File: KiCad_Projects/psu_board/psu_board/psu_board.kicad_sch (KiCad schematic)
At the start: 23 parts, among them J1 Conn_01x02_Female, J2 Conn_01x02_Female, J3 Conn_01x02_Female, SW1 SW_DIP_x01, SW2 SW_DIP_x01, U1 OKL-T_6-W12N-C

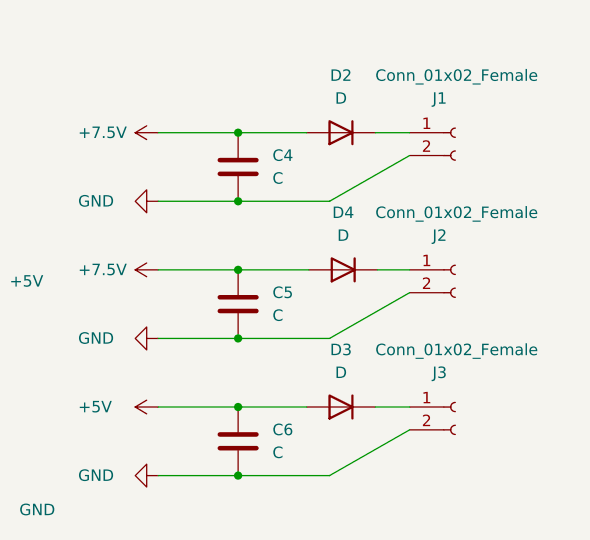
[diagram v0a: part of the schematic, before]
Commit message: 基盤データのアップデート
ローカルコミットはちゃんと作ってください
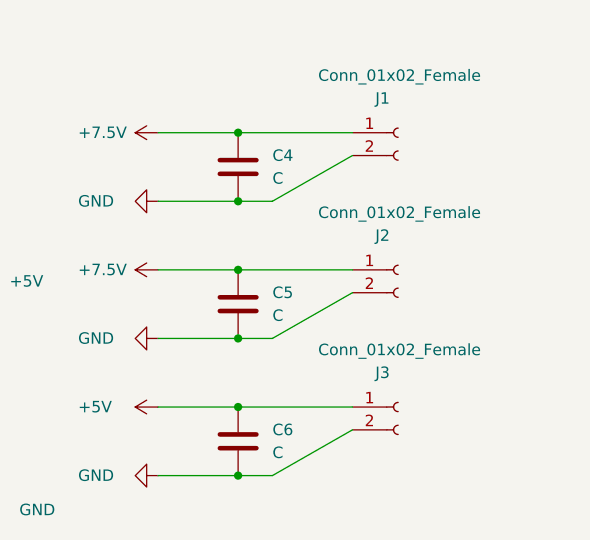
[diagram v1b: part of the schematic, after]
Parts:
- removed D2, D3, D4: D, Diode_THT:D_DO-41_SOD81_P7.62mm_Horizontal, symbol Device:D
- BT1: footprint (none) -> Connector_JST:JST_VH_B2P-VH-B_1x02_P3.96mm_Vertical
- C6: footprint Capacitor_THT:CP_Radial_D5.0mm_P2.50mm -> (none)
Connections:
- net +5V: now also J3.1 (Pin_1)
- net +7.5V: now also J1.1 (Pin_1), J2.1 (Pin_1)
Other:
- moved on the sheet: J1, J2, J3
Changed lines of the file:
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@@
-    (stroke (width 0) (type default) (color 0 0 0 0))
-  )
-  (wire (pts (xy 236.22 110.49) (xy 240.03 110.49))
     (stroke (width 0) (type default) (color 0 0 0 0))
   )
@@
     (stroke (width 0) (type default) (color 0 0 0 0))
   )
-  (wire (pts (xy 220.98 102.87) (xy 231.14 102.87))
-    (stroke (width 0) (type default) (color 0 0 0 0))
-  )
-  (wire (pts (xy 220.98 80.01) (xy 228.6 80.01))
+  (wire (pts (xy 220.98 102.87) (xy 224.79 102.87))
     (stroke (width 0) (type default) (color 0 0 0 0))
   )
@@
     (stroke (width 0) (type default) (color 0 0 0 0))
   )
-  (wire (pts (xy 236.4672 95.25) (xy 240.03 95.25))
-    (stroke (width 0) (type default) (color 0 0 0 0))
-  )
   (wire (pts (xy 109.22 105.41) (xy 109.22 101.6))
     (stroke (width 0) (type default) (color 0 0 0 0))
@@
     (stroke (width 0) (type default) (color 0 0 0 0))
   )
-  (wire (pts (xy 231.14 102.87) (xy 240.03 97.79))
+  (wire (pts (xy 224.79 102.87) (xy 233.68 97.79))
     (stroke (width 0) (type default) (color 0 0 0 0))
   )
@@
     (stroke (width 0) (type default) (color 0 0 0 0))
   )
-  (wire (pts (xy 220.98 110.49) (xy 228.6 110.49))
+  (wire (pts (xy 220.98 110.49) (xy 233.68 110.49))
     (stroke (width 0) (type default) (color 0 0 0 0))
   )
@@
     (stroke (width 0) (type default) (color 0 0 0 0))
   )
-  (wire (pts (xy 231.14 87.63) (xy 240.03 82.55))
+  (wire (pts (xy 224.79 87.63) (xy 233.68 82.55))
     (stroke (width 0) (type default) (color 0 0 0 0))
   )
@@
     (stroke (width 0) (type default) (color 0 0 0 0))
   )
-  (wire (pts (xy 231.14 118.11) (xy 240.03 113.03))
-    (stroke (width 0) (type default) (color 0 0 0 0))
-  )
-  (wire (pts (xy 220.98 95.25) (xy 228.8472 95.25))
+  (wire (pts (xy 224.79 118.11) (xy 233.68 113.03))
+    (stroke (width 0) (type default) (color 0 0 0 0))
+  )
+  (wire (pts (xy 220.98 95.25) (xy 233.68 95.25))
     (stroke (width 0) (type default) (color 0 0 0 0))
   )
@@
     (stroke (width 0) (type default) (color 0 0 0 0))
   )
-  (wire (pts (xy 236.22 80.01) (xy 240.03 80.01))
+  (wire (pts (xy 220.98 80.01) (xy 233.68 80.01))
     (stroke (width 0) (type default) (color 0 0 0 0))
   )
@@
     (stroke (width 0) (type default) (color 0 0 0 0))
   )
-  (wire (pts (xy 220.98 87.63) (xy 231.14 87.63))
+  (wire (pts (xy 220.98 87.63) (xy 224.79 87.63))
     (stroke (width 0) (type default) (color 0 0 0 0))
   )
@@
     (stroke (width 0) (type default) (color 0 0 0 0))
   )
-  (wire (pts (xy 220.98 118.11) (xy 231.14 118.11))
+  (wire (pts (xy 220.98 118.11) (xy 224.79 118.11))
     (stroke (width 0) (type default) (color 0 0 0 0))
   )
@@
       (effects (font (size 1.27 1.27)) (justify left))
     )
-    (property "Footprint" "" (id 2) (at 80.01 79.756 90)
+    (property "Footprint" "Connector_JST:JST_VH_B2P-VH-B_1x02_P3.96mm_Vertical" (id 2) (at 80.01 79.756 90)
       (effects (font (size 1.27 1.27)) hide)
     )
     (property "Datasheet" "~" (id 3) (at 80.01 79.756 90)
-      (effects (font (size 1.27 1.27)) hide)
-    )
-    (pin "1")
-    (pin "2")
-  )
-  (symbol (lib_id "Device:D") (at 232.41 80.01 180) (unit 1)
-    (in_bom yes) (on_board yes) (fields_autoplaced)
-    (property "Reference" "D2" (id 0) (at 232.41 73.66 0))
-    (property "Value" "D" (id 1) (at 232.41 76.2 0))
-    (property "Footprint" "Diode_THT:D_DO-41_SOD81_P7.62mm_Horizontal" (id 2) (at 232.41 80.01 0)
-      (effects (font (size 1.27 1.27)) hide)
-    )
-    (property "Datasheet" "~" (id 3) (at 232.41 80.01 0)
       (effects (font (size 1.27 1.27)) hide)
     )
@@
     (pin "1")
   )
-  (symbol (lib_id "Device:D") (at 232.6572 95.25 180) (unit 1)
-    (in_bom yes) (on_board yes) (fields_autoplaced)
-    (property "Reference" "D4" (id 0) (at 232.6572 88.9 0))
-    (property "Value" "D" (id 1) (at 232.6572 91.44 0))
-    (property "Footprint" "Diode_THT:D_DO-41_SOD81_P7.62mm_Horizontal" (id 2) (at 232.6572 95.25 0)
-      (effects (font (size 1.27 1.27)) hide)
-    )
-    (property "Datasheet" "~" (id 3) (at 232.6572 95.25 0)
-      (effects (font (size 1.27 1.27)) hide)
-    )
-    (pin "1")
-    (pin "2")
-  )
   (symbol (lib_id "Device:C") (at 220.98 99.06 0) (unit 1)
     (in_bom yes) (on_board yes) (fields_autoplaced)
@@
       (effects (font (size 1.27 1.27)) (justify left))
     )
-    (property "Footprint" "Capacitor_THT:CP_Radial_D5.0mm_P2.50mm" (id 2) (at 221.9452 118.11 0)
+    (property "Footprint" "" (id 2) (at 221.9452 118.11 0)
       (effects (font (size 1.27 1.27)) hide)
     )
@@
     (pin "2")
   )
-  (symbol (lib_id "Connector:Conn_01x02_Female") (at 245.11 95.25 0) (unit 1)
-    (in_bom yes) (on_board yes)
-    (property "Reference" "J2" (id 0) (at 242.57 91.44 0)
-      (effects (font (size 1.27 1.27)) (justify left))
-    )
-    (property "Value" "Conn_01x02_Female" (id 1) (at 236.22 88.9 0)
-      (effects (font (size 1.27 1.27)) (justify left))
-    )
-    (property "Footprint" "Connector_PinSocket_2.54mm:PinSocket_1x02_P2.54mm_Vertical" (id 2) (at 245.11 95.25 0)
-      (effects (font (size 1.27 1.27)) hide)
-    )
-    (property "Datasheet" "~" (id 3) (at 245.11 95.25 0)
+  (symbol (lib_id "Connector:Conn_01x02_Female") (at 238.76 95.25 0) (unit 1)
+    (in_bom yes) (on_board yes)
+    (property "Reference" "J2" (id 0) (at 236.22 91.44 0)
+      (effects (font (size 1.27 1.27)) (justify left))
+    )
+    (property "Value" "Conn_01x02_Female" (id 1) (at 229.87 88.9 0)
+      (effects (font (size 1.27 1.27)) (justify left))
+    )
+    (property "Footprint" "Connector_PinSocket_2.54mm:PinSocket_1x02_P2.54mm_Vertical" (id 2) (at 238.76 95.25 0)
+      (effects (font (size 1.27 1.27)) hide)
+    )
+    (property "Datasheet" "~" (id 3) (at 238.76 95.25 0)
       (effects (font (size 1.27 1.27)) hide)
     )
@@
     (pin "1")
   )
-  (symbol (lib_id "Device:D") (at 232.41 110.49 180) (unit 1)
-    (in_bom yes) (on_board yes) (fields_autoplaced)
-    (property "Reference" "D3" (id 0) (at 232.41 104.14 0))
-    (property "Value" "D" (id 1) (at 232.41 106.68 0))
-    (property "Footprint" "Diode_THT:D_DO-41_SOD81_P7.62mm_Horizontal" (id 2) (at 232.41 110.49 0)
-      (effects (font (size 1.27 1.27)) hide)
-    )
-    (property "Datasheet" "~" (id 3) (at 232.41 110.49 0)
-      (effects (font (size 1.27 1.27)) hide)
-    )
-    (pin "1")
-    (pin "2")
-  )
   (symbol (lib_id "power:GND") (at 212.09 118.11 270) (unit 1)
     (in_bom yes) (on_board yes)
@@
     (pin "1")
   )
-  (symbol (lib_id "Connector:Conn_01x02_Female") (at 245.11 80.01 0) (unit 1)
-    (in_bom yes) (on_board yes)
-    (property "Reference" "J1" (id 0) (at 242.57 76.2 0)
-      (effects (font (size 1.27 1.27)) (justify left))
-    )
-    (property "Value" "Conn_01x02_Female" (id 1) (at 236.22 73.66 0)
-      (effects (font (size 1.27 1.27)) (justify left))
-    )
-    (property "Footprint" "Connector_PinSocket_2.54mm:PinSocket_1x02_P2.54mm_Vertical" (id 2) (at 245.11 80.01 0)
-      (effects (font (size 1.27 1.27)) hide)
-    )
-    (property "Datasheet" "~" (id 3) (at 245.11 80.01 0)
+  (symbol (lib_id "Connector:Conn_01x02_Female") (at 238.76 80.01 0) (unit 1)
+    (in_bom yes) (on_board yes)
+    (property "Reference" "J1" (id 0) (at 236.22 76.2 0)
+      (effects (font (size 1.27 1.27)) (justify left))
+    )
+    (property "Value" "Conn_01x02_Female" (id 1) (at 229.87 73.66 0)
+      (effects (font (size 1.27 1.27)) (justify left))
+    )
+    (property "Footprint" "Connector_PinSocket_2.54mm:PinSocket_1x02_P2.54mm_Vertical" (id 2) (at 238.76 80.01 0)
+      (effects (font (size 1.27 1.27)) hide)
+    )
+    (property "Datasheet" "~" (id 3) (at 238.76 80.01 0)
       (effects (font (size 1.27 1.27)) hide)
     )
@@
     (pin "1")
   )
-  (symbol (lib_id "Connector:Conn_01x02_Female") (at 245.11 110.49 0) (unit 1)
-    (in_bom yes) (on_board yes)
-    (property "Reference" "J3" (id 0) (at 242.57 106.68 0)
-      (effects (font (size 1.27 1.27)) (justify left))
-    )
-    (property "Value" "Conn_01x02_Female" (id 1) (at 236.22 104.14 0)
-      (effects (font (size 1.27 1.27)) (justify left))
-    )
-    (property "Footprint" "Connector_PinSocket_2.54mm:PinSocket_1x02_P2.54mm_Vertical" (id 2) (at 245.11 110.49 0)
-      (effects (font (size 1.27 1.27)) hide)
-    )
-    (property "Datasheet" "~" (id 3) (at 245.11 110.49 0)
+  (symbol (lib_id "Connector:Conn_01x02_Female") (at 238.76 110.49 0) (unit 1)
+    (in_bom yes) (on_board yes)
+    (property "Reference" "J3" (id 0) (at 236.22 106.68 0)
+      (effects (font (size 1.27 1.27)) (justify left))
+    )
+    (property "Value" "Conn_01x02_Female" (id 1) (at 229.87 104.14 0)
+      (effects (font (size 1.27 1.27)) (justify left))
+    )
+    (property "Footprint" "Connector_PinSocket_2.54mm:PinSocket_1x02_P2.54mm_Vertical" (id 2) (at 238.76 110.49 0)
+      (effects (font (size 1.27 1.27)) hide)
+    )
+    (property "Datasheet" "~" (id 3) (at 238.76 110.49 0)
       (effects (font (size 1.27 1.27)) hide)
     )
@@
     )
     (path "/5f65e910-0e23-4454-ab02-e2c41faaf4ed"
-      (reference "C6") (unit 1) (value "C") (footprint "Capacitor_THT:CP_Radial_D5.0mm_P2.50mm")
+      (reference "C6") (unit 1) (value "C") (footprint "Capacitor_THT:C_Disc_D3.8mm_W2.6mm_P2.50mm")
     )
     (path "/cdbea2fa-6a53-4cd6-92f6-062ed9028ff4"
       (reference "D1") (unit 1) (value "D_Shockley") (footprint "Diode_THT:D_5W_P10.16mm_Horizontal")
     )
-    (path "/1d671dab-7070-485b-8f55-0effa957e3b0"
-      (reference "D2") (unit 1) (value "D") (footprint "Diode_THT:D_DO-41_SOD81_P7.62mm_Horizontal")
-    )
-    (path "/88ac9789-8ce6-4dfc-afc8-c57f0bf12e81"
-      (reference "D3") (unit 1) (value "D") (footprint "Diode_THT:D_DO-41_SOD81_P7.62mm_Horizontal")
-    )
-    (path "/40c9d126-34a3-4c5f-80af-3321809da666"
-      (reference "D4") (unit 1) (value "D") (footprint "Diode_THT:D_DO-41_SOD81_P7.62mm_Horizontal")
-    )
     (path "/2197c9be-58d1-4c42-8c39-5759355f3cec"
